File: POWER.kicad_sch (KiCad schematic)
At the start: 43 parts, among them U4 LFMXO5-25

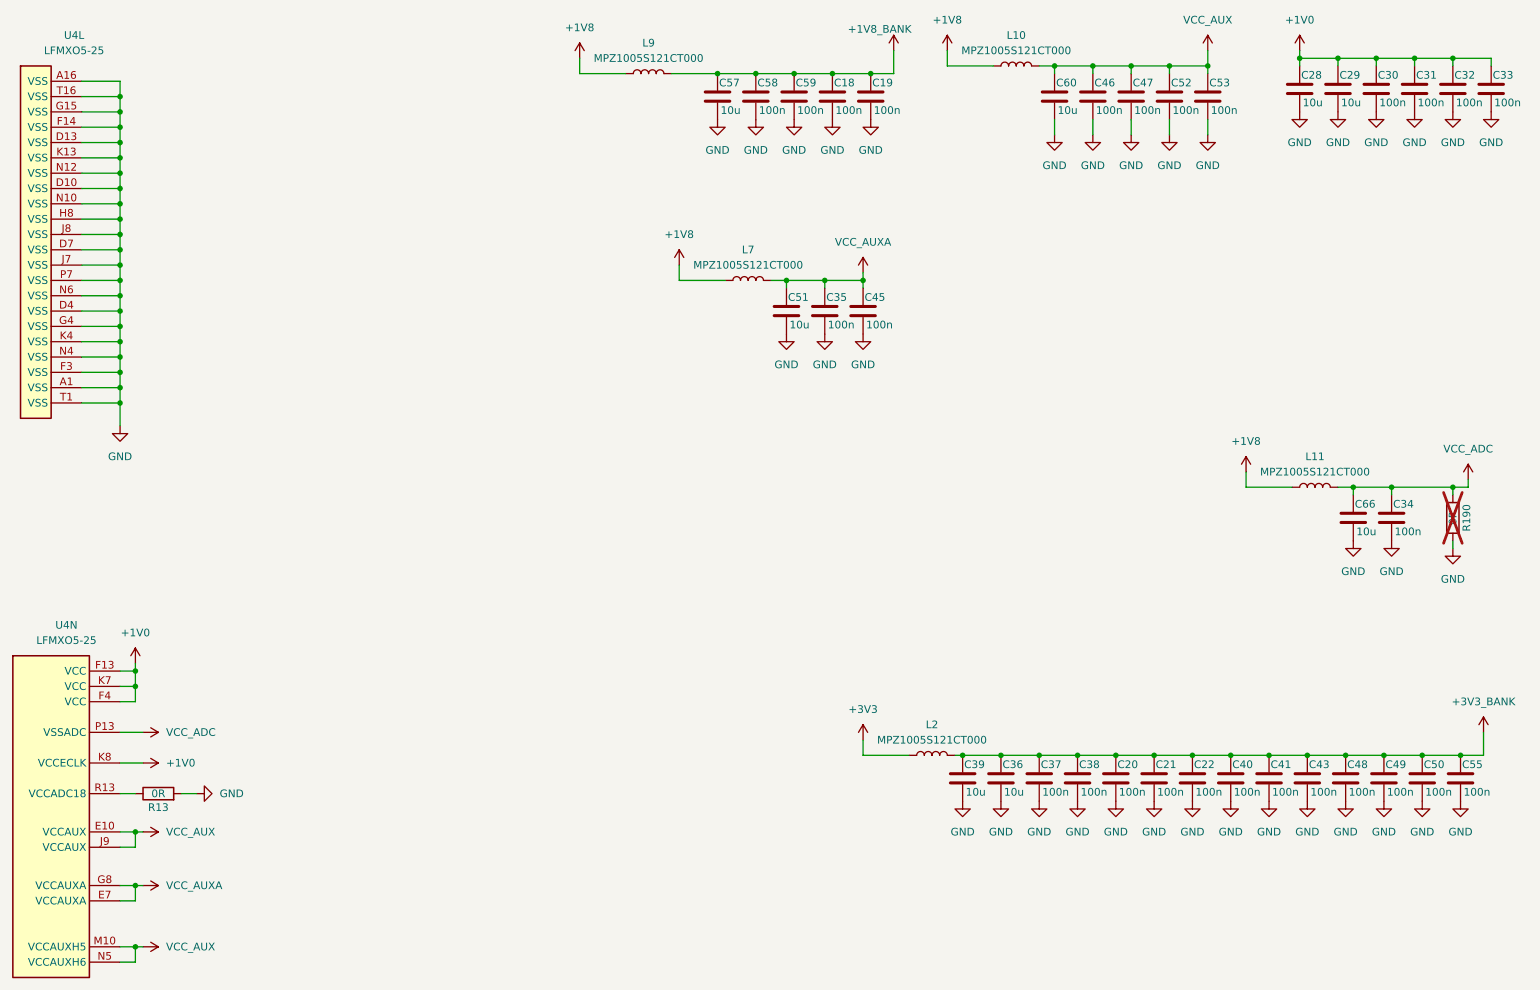
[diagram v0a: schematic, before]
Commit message: relay unit
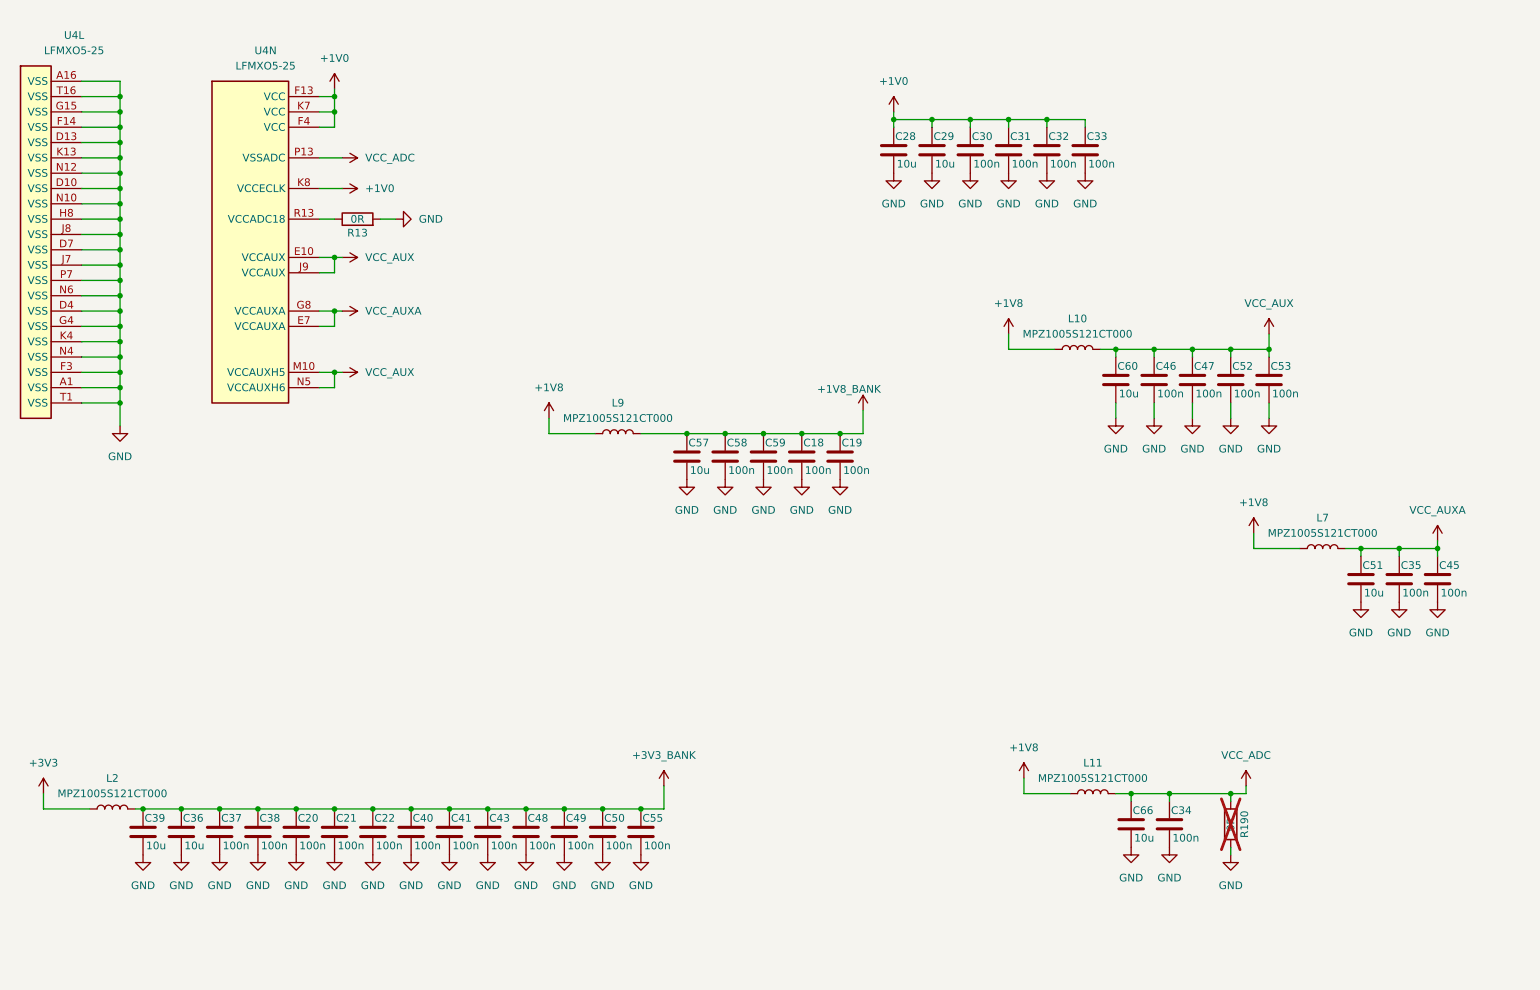
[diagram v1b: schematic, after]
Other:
- moved on the sheet: C18, C19, C20, C21, C22, C28, C29, C30, C31, C32, C33, C34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
